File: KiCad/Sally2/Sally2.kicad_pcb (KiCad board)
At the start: 2 copper layers, 220 x 150 mm, 76 parts, among them J1 Power SW, J10 GND +5V, J11 A16, J12 Drive 1-4, J13 OPT, J14 Special_Func, J15 TX GND RX, J16 + RI -, J17 RS232, J18 IN RDY CMD OUT GND, J19 Centronics, J2 Power LED, J20 Conn_01x13, J3 USB_B, J4 PowerIn, J5 GND +5V, J6 Barrel_Jack, J7 GND +5V, J8 Conn_01x13, J9 + A14 -, SW1 Reset, U1 GAL16V8 - IO decoder, U10 MAX232, U11 74LS06, U12 74LS06, U13 Z84C30, U14 74LS244, U15 74LS273, U16 74LS244, U2 Z80ACPU, U3 GAL16V8 - ADR decoder, U4 27C256, U5 628128_DIP32_SSOP32, U6 GAL16V8 - glue logic, U7 74LS259, U8 74LS273, U9 WD1772_PHY, X1 16Mhz

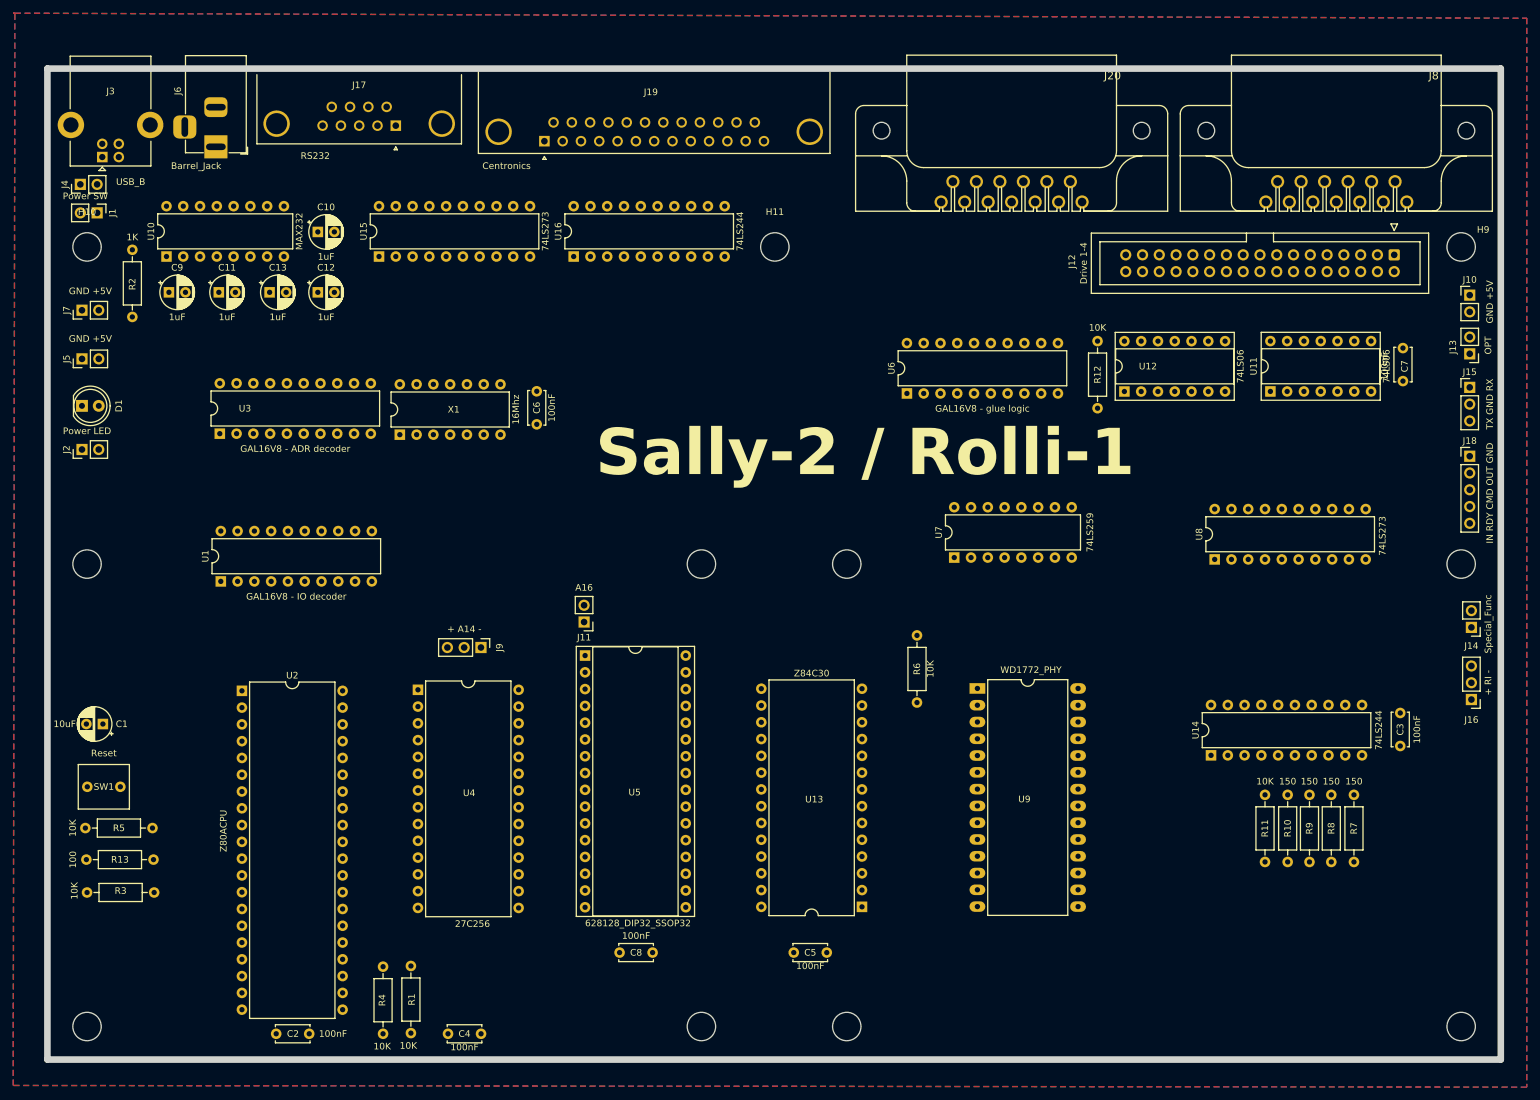
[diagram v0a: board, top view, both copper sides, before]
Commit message: KiCad merges from Marc
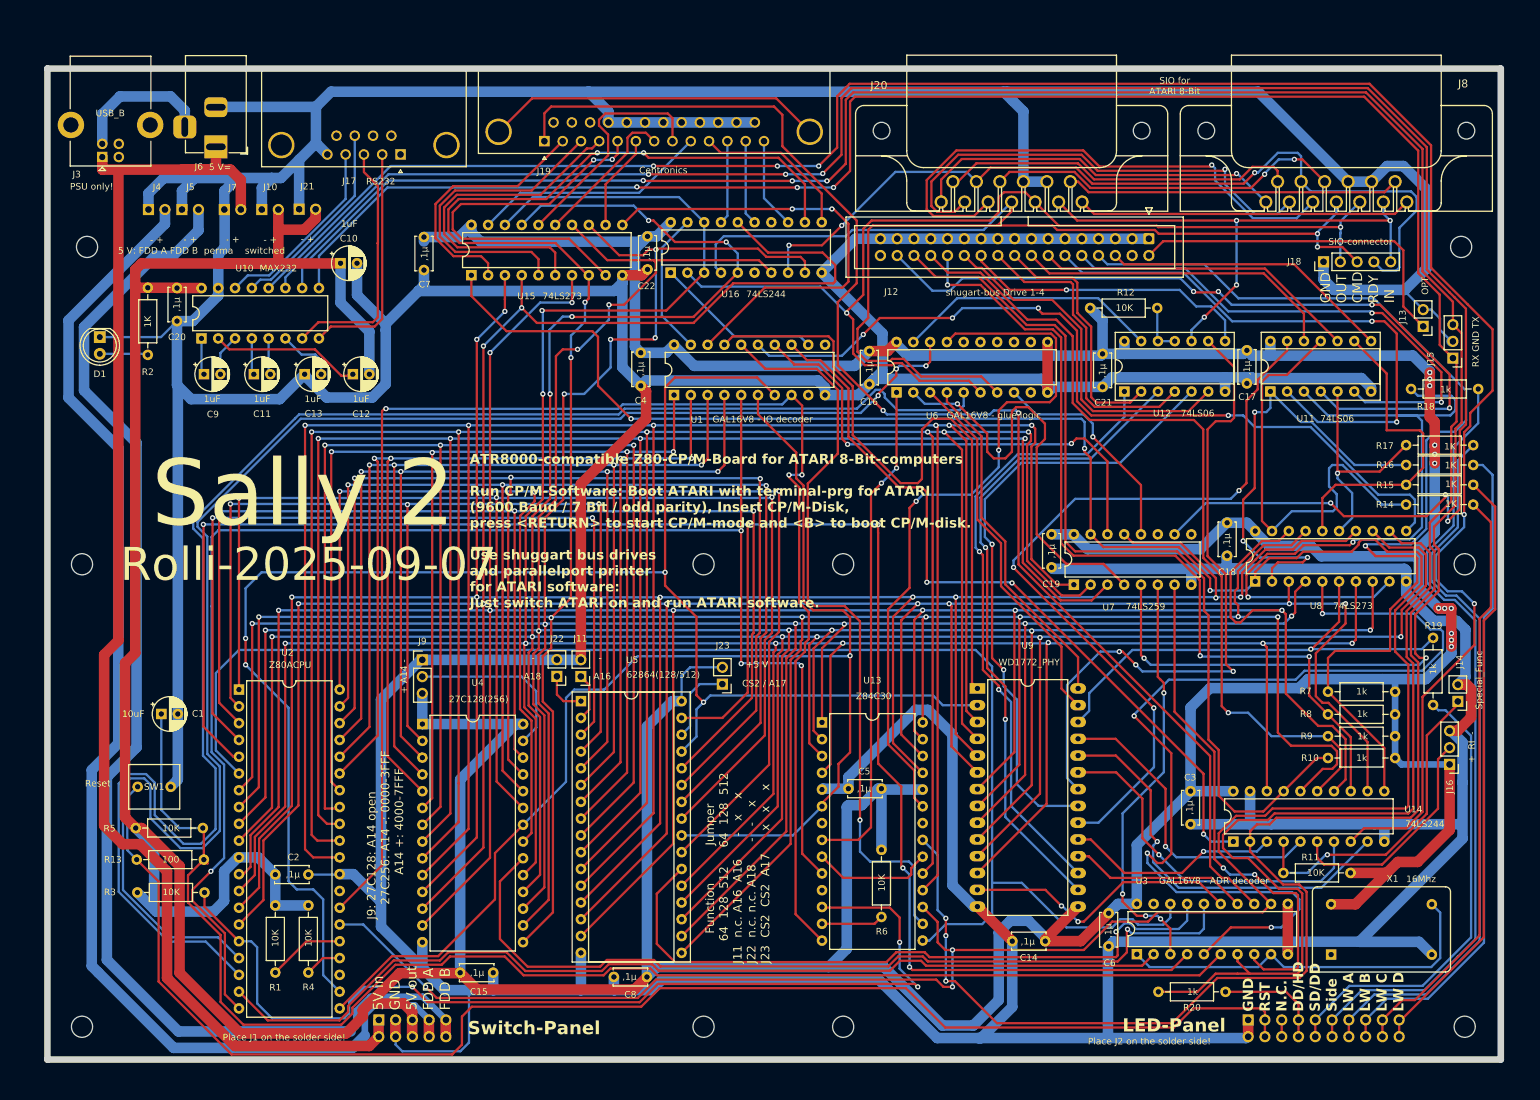
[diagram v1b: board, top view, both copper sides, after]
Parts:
- removed H11: MountingHole, MountingHole:MountingHole_4.3mm_M4
- added C14: ,1µ, Capacitor_THT:C_Disc_D5.0mm_W2.5mm_P5.00mm, F.Cu at (161.0, 132.1)
- added C15: ,1µ, Capacitor_THT:C_Disc_D5.0mm_W2.5mm_P5.00mm, F.Cu at (72.5, 136.9)
- added C16: ,1µ, Capacitor_THT:C_Disc_D5.0mm_W2.5mm_P5.00mm, F.Cu at (134.4, 42.8)
- added C17: ,1µ, Capacitor_THT:C_Disc_D5.0mm_W2.5mm_P5.00mm, F.Cu at (191.6, 42.7)
- added C18: ,1µ, Capacitor_THT:C_Disc_D5.0mm_W2.5mm_P5.00mm, F.Cu at (188.6, 68.8)
- added C19: ,1µ, Capacitor_THT:C_Disc_D5.0mm_W2.5mm_P5.00mm, F.Cu at (162.0, 70.5)
- added C20: ,1µ, Capacitor_THT:C_Disc_D5.0mm_W2.5mm_P5.00mm, F.Cu at (29.6, 33.2)
- added C21: ,1µ, Capacitor_THT:C_Disc_D5.0mm_W2.5mm_P5.00mm, F.Cu at (169.7, 43.2)
- added C22: ,1µ, Capacitor_THT:C_Disc_D5.0mm_W2.5mm_P5.00mm, F.Cu at (100.8, 25.4)
- added J21: - +, Sally2:BKL_1x2 72510U_P2.5mm_Vertical, F.Cu at (49.4, 21.2)
- added J22: A18, Connector_PinHeader_2.54mm:PinHeader_1x02_P2.54mm_Vertical, F.Cu at (87.1, 92.0)
- added J23: CS2 / A17, Connector_PinHeader_2.54mm:PinHeader_1x02_P2.54mm_Vertical, F.Cu at (112.2, 93.2)
- added R14: 1K, Resistor_THT:R_Axial_DIN0207_L6.3mm_D2.5mm_P10.16mm_Horizontal, F.Cu at (225.8, 66.0)
- added R15: 1K, Resistor_THT:R_Axial_DIN0207_L6.3mm_D2.5mm_P10.16mm_Horizontal, F.Cu at (225.8, 63.0)
- added R16: 1K, Resistor_THT:R_Axial_DIN0207_L6.3mm_D2.5mm_P10.16mm_Horizontal, F.Cu at (225.8, 60.0)
- added R17: 1K, Resistor_THT:R_Axial_DIN0207_L6.3mm_D2.5mm_P10.16mm_Horizontal, F.Cu at (225.8, 57.0)
- added R18: 1k, Resistor_THT:R_Axial_DIN0207_L6.3mm_D2.5mm_P10.16mm_Horizontal, F.Cu at (226.6, 48.5)
- added R19: 1k, Resistor_THT:R_Axial_DIN0207_L6.3mm_D2.5mm_P10.16mm_Horizontal, F.Cu at (219.8, 96.3)
- added R20: 1k, Resistor_THT:R_Axial_DIN0207_L6.3mm_D2.5mm_P10.16mm_Horizontal, F.Cu at (188.3, 139.8)
- C2, C3, C4, C5, C6, C7, C8: value 100nF -> ,1µ
- H1, H10, H2, H3, H4, H5, H6, H7, H8, H9: footprint MountingHole:MountingHole_4.3mm_M4 -> MountingHole:MountingHole_3.2mm_M3
- J1: value Power SW -> Conn_02x05_Odd_Even; footprint Connector_PinHeader_2.54mm:PinHeader_1x02_P2.54mm_Vertical -> Connector_PinHeader_2.54mm:PinHeader_2x05_P2.54mm_Horizontal; moved to B.Cu
- J10, J5, J7: value GND +5V -> - +; footprint Connector_PinHeader_2.54mm:PinHeader_1x02_P2.54mm_Vertical -> Sally2:BKL_1x2 72510U_P2.5mm_Vertical
- J12: value Drive 1-4 -> shugart-bus Drive 1-4
- J15: value TX GND RX -> RX GND TX
- J16: value + RI - -> + RI -
- J17: footprint Connector_Dsub:DSUB-9_Male_Horizontal_P2.77x2.84mm_EdgePinOffset4.94mm_Housed_MountingHolesOffset7.48mm -> Connector_Dsub:DSUB-9_Male_Horizontal_P2.77x2.84mm_EdgePinOffset9.90mm_Housed_MountingHolesOffset11.32mm
- J18: value IN RDY CMD OUT GND -> SIO-connector
- J2: value Power LED -> Conn_02x10_Odd_Even; footprint Connector_PinHeader_2.54mm:PinHeader_1x02_P2.54mm_Vertical -> Connector_PinHeader_2.54mm:PinHeader_2x10_P2.54mm_Horizontal; moved to B.Cu
- J4: value PowerIn -> - +; footprint Connector_PinHeader_2.54mm:PinHeader_1x02_P2.54mm_Vertical -> Sally2:BKL_1x2 72510U_P2.5mm_Vertical
- R10, R7, R8, R9: value 150 -> 1k
- U4: value 27C256 -> 27C128(256)
- U5: value 628128_DIP32_SSOP32 -> 62864(128/512)
- X1: footprint Package_DIP:DIP-14_W7.62mm -> Oscillator:Oscillator_DIP-14
- moved J2 196.5 mm to (191.8, 144.0), turned to -90 degrees
- moved J10 182.0 mm to (43.7, 21.3), turned to -90 degrees
- moved X1 161.5 mm to (204.3, 134.1), turned to 0 degrees
- moved U3 159.6 mm to (174.9, 134.1)
- moved C7 149.1 mm to (67.0, 25.5)
- moved J1 129.4 mm to (60.2, 144.0)
- moved C6 117.2 mm to (170.6, 127.9)
- moved C4 107.1 mm to (99.8, 43.0), turned to -90 degrees
- moved U1 74.2 mm to (104.9, 49.4)
- moved J12 37.2 mm to (176.7, 25.8)
- moved J18 36.8 mm to (203.2, 29.2), turned to 90 degrees
- moved C3 33.9 mm to (183.0, 109.4)
- moved R6 32.9 mm to (136.2, 118.2)
- moved U13 28.6 mm to (127.2, 99.0), turned to 0 degrees
- moved R1 28.2 mm to (44.5, 126.7), turned to -90 degrees
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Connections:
- J1 pad 1: +5V -> Net-(J1-Pin_1)
- J1 pad 2: Net-(J1-Pin_2) -> Net-(J1-Pin_1)
- J2 pad 2: Net-(D1-A) -> GND
- J3 pad 1: Net-(J1-Pin_2) -> Net-(J1-Pin_1)
- J3 pad 4: GND -> Net-(J3-GND)
- J4 pad 2: Net-(J1-Pin_2) -> Net-(J1-Pin_7)
- J5 pad 2: +5V -> Net-(J1-Pin_10)
- J6 pad 1: Net-(J1-Pin_2) -> Net-(J1-Pin_1)
- J6 pad 3: unconnected-(J6-MountPin-Pad3) -> Net-(J3-GND)
- J7 pad 2: +5V -> Net-(J1-Pin_1)
- R13 pad 2: Net-(R13-Pad2) -> RES SW
- SW1 pad 2: Net-(R13-Pad2) -> RES SW
- U5 pad 1: unconnected-(U5-NC-Pad1) -> Net-(J22-Pin_1)
- U5 pad 30: +5V -> Net-(J23-Pin_1)
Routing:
- net GND: track 0.00 -> 1415.4 mm
- net +5V: track 0.00 -> 1063.4 mm, vias 0 -> 12
- net D3: track 0.00 -> 546.3 mm, vias 0 -> 11
- net D1: track 0.00 -> 527.2 mm, vias 0 -> 9
- net D7: track 0.00 -> 493.2 mm, vias 0 -> 9
- net D6: track 0.00 -> 490.5 mm, vias 0 -> 10
- net A0: track 0.00 -> 471.9 mm, vias 0 -> 6
- net D2: track 0.00 -> 471.8 mm, vias 0 -> 8
- net A1: track 0.00 -> 459.8 mm, vias 0 -> 6
- net D5: track 0.00 -> 453.7 mm, vias 0 -> 8
- net D4: track 0.00 -> 449.1 mm, vias 0 -> 10
- net D0: track 0.00 -> 441.8 mm, vias 0 -> 9
- net RESC\: track 0.00 -> 435.0 mm, vias 0 -> 6
- net RX: track 0.00 -> 433.2 mm, vias 0 -> 6
- net TX: track 0.00 -> 332.1 mm, vias 0 -> 5
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- removed copper zone on B.Cu, net GND
- removed copper zone on F.Cu, net GND
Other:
- board text added: "+5 V"
- board text added: "-"
- board text added: "5 V: FDD A FDD B perma switched"
- board text added: "5 V="
- board text added: "5V in GND 5V out FDD A FDD B"
- board text added: "ATR8000-compatible Z80-CP/M-Board for ATARI 8-Bit-computers Run CP/M-Software: Boot ATARI with terminal-prg for ATARI (9600 Baud / 7 Bit / odd parity), Insert CP/M-Disk, press <RETURN> to start CP/M-mode and <B> to boot CP/M-disk. Use shuggart bus drives and parallelport printer for ATARI software: Just switch ATARI on and run ATARI software."
- board text added: "Function Jumper 64 128 512 64 128 512 J11 n.c. A16 A16 - x x J22 n.c. n.c. A18 - - x J23 CS2 CS2 A17 x x x"
- board text added: "GND OUT CMD RDY IN"
- board text added: "GND RST N.C. DD/HD SD/DD Side LW A LW B LW C LW D"
- board text added: "J9: 27C128: A14 open 27C256: A14 -: 0000-3FFF A14 +: 4000-7FFF"
- board text added: "LED-Panel"
- board text added: "PSU only!"
- board text added: "Place J1 on the solder side!"
- board text added: "Place J2 on the solder side!"
- board text added: "Rolli-2025-09-07"
- board text added: "SIO for ATARI 8-Bit"
- board text added: "Sally 2"
- board text added: "Switch-Panel"
- board text removed: "Sally-2 / Rolli-1"
